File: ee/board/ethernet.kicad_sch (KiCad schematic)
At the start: 20 parts, among them J8 HR911105A, U1 RTL8201F, Y1 Crystal_GND24_Small

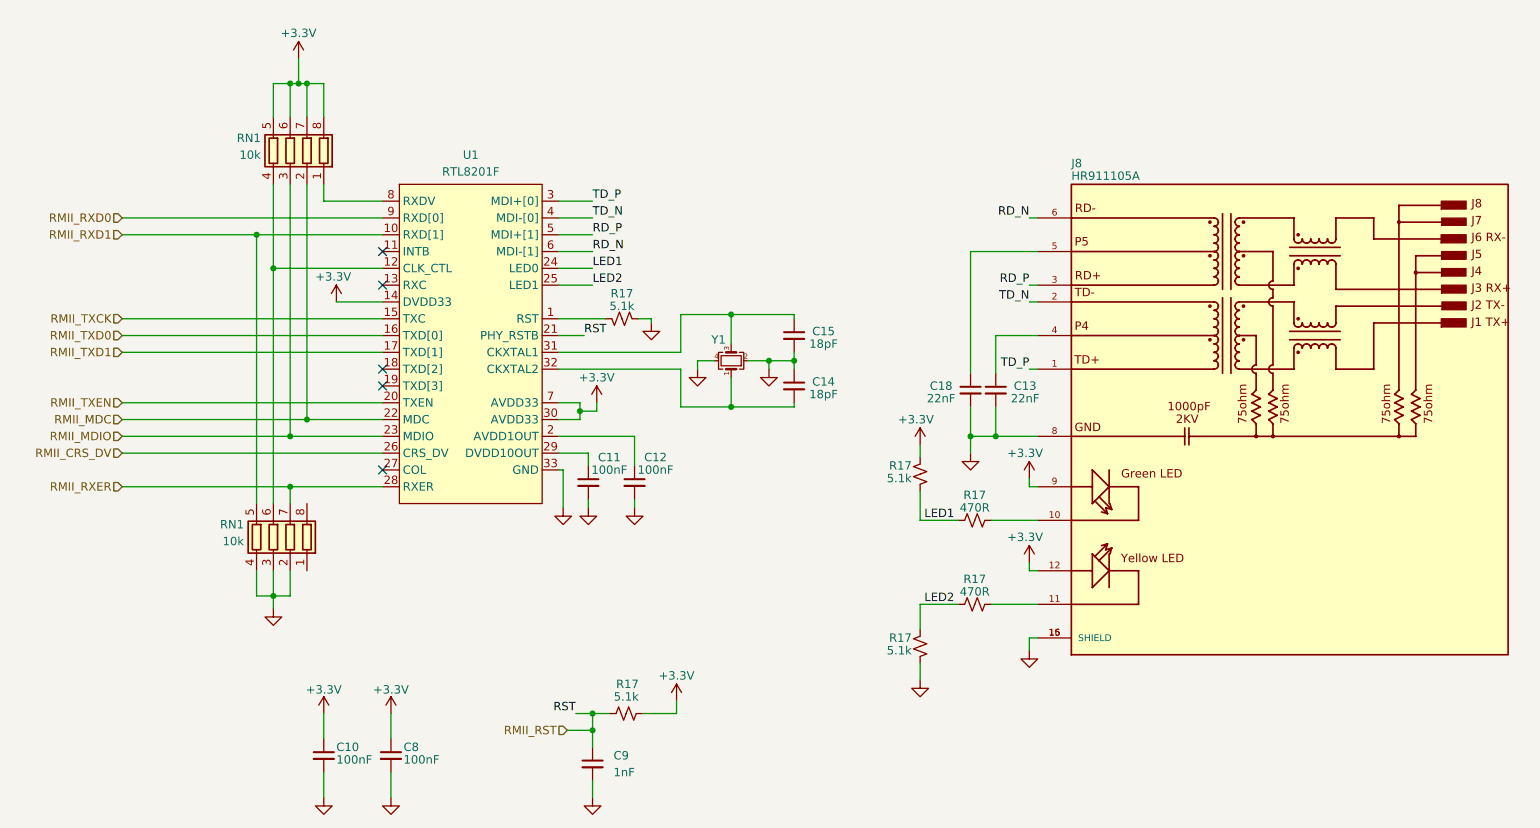
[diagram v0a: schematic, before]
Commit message: Nearly finished routing.
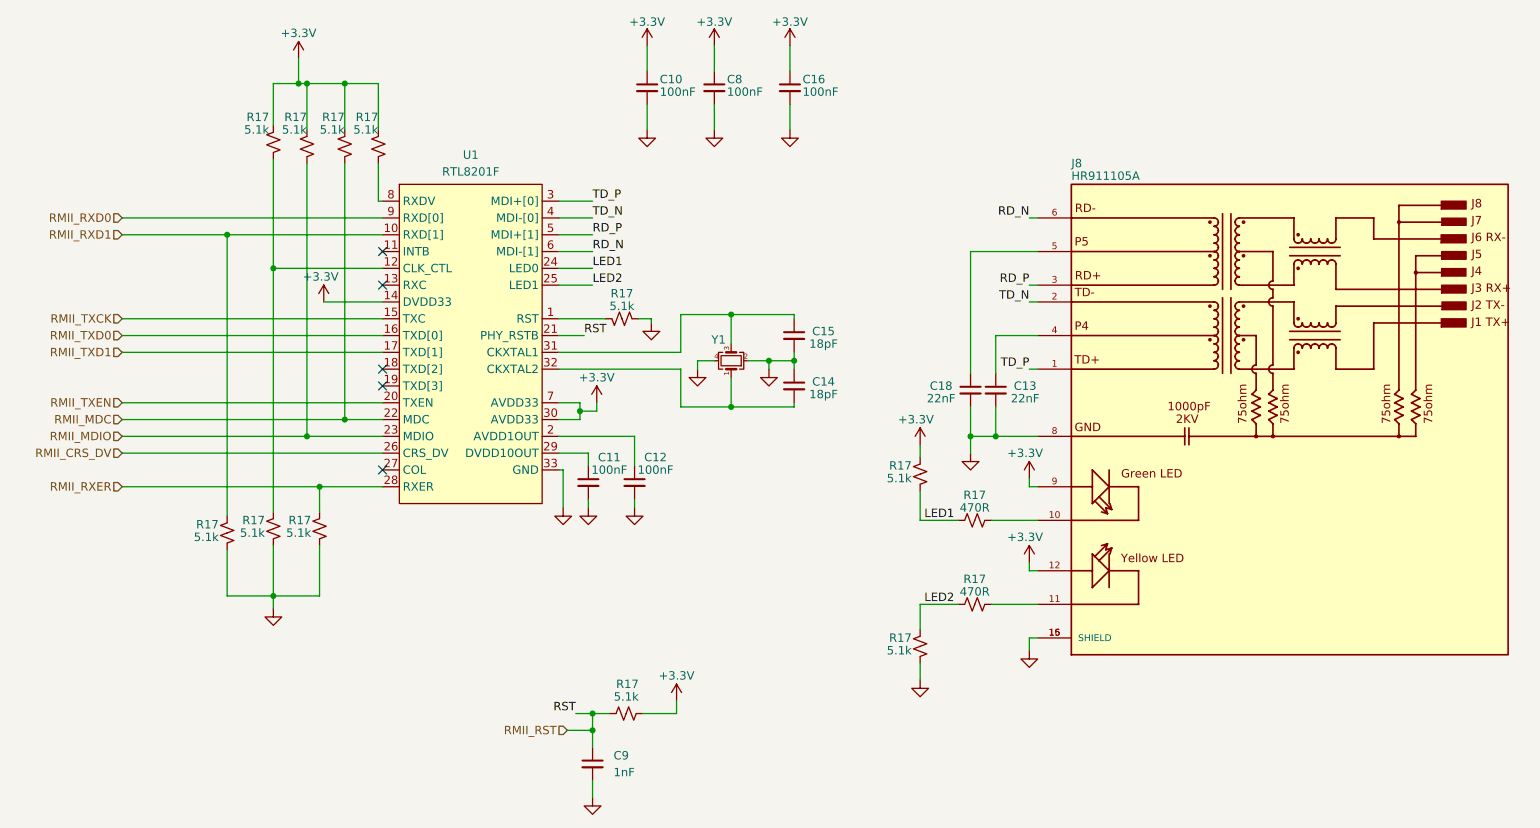
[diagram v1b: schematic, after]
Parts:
- removed RN1 (x2): 10k, Resistor_SMD:R_Array_Convex_4x0402, symbol Device:R_Pack04
- added C16: 100nF, Capacitor_SMD:C_0603_1608Metric, symbol Device:C_Small
- added R17 (x7): 5.1k, Resistor_SMD:R_0603_1608Metric, symbol Device:R_Small_US
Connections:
- net +3V3: now also C16.1, R17.2, R17.2, R17.2, R17.2
- net GND: now also C16.2, R17.1, R17.1, R17.1
- net RMII_MDC: now also R17.1
- net RMII_MDIO: now also R17.1
- net RMII_RXD1: now also R17.2
- net RMII_RXER: now also R17.2
- net at U1.12 (CLK_CTL): now also R17.1, R17.2
- net at U1.8 (RXDV): now also R17.1
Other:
- moved on the sheet: C10, C8

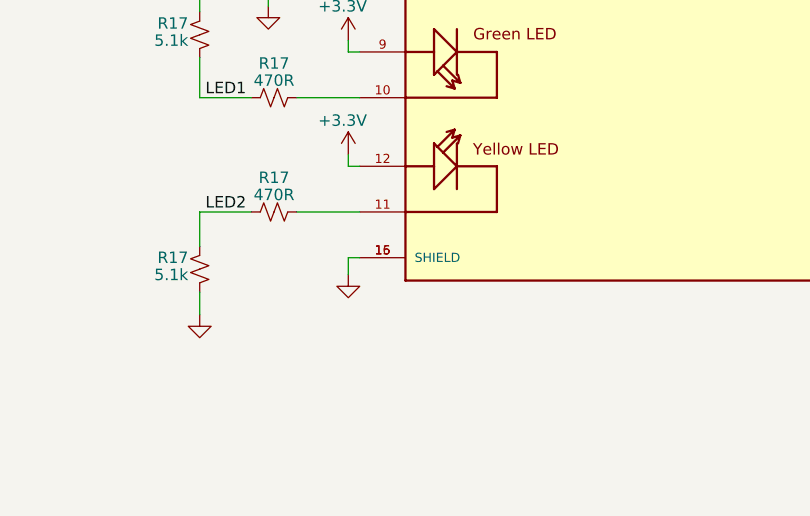
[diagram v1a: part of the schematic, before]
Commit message: Finished R1
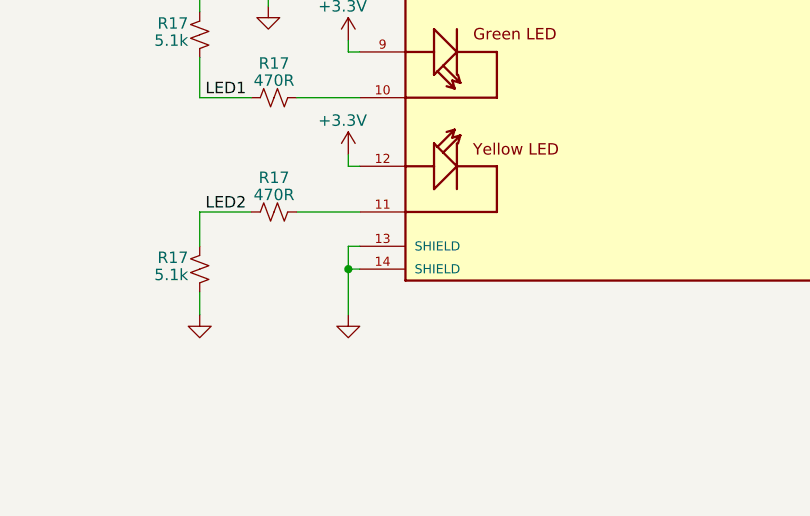
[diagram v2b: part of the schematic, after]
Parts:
- C10, C11, C12, C16, C8: MPN (none) -> CC0603KRX7R7BB104
- C14, C15: MPN (none) -> CC0603JPNPO9BN180
- R17: MPN (none) -> RC0603FR-135K1L
- R17: MPN (none) -> RC0603FR-13470KL
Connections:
- net GND: now also J8.13 (SHIELD), J8.14 (SHIELD); no longer J8.15 (SHIELD), J8.16 (SHIELD)
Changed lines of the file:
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@@
   (junction (at 86.995 90.17) (diameter 0) (color 0 0 0 0)
+  )
+  (junction (at 190.5 124.46) (diameter 0) (color 0 0 0 0)
   )
   (junction (at 83.185 100.33) (diameter 0) (color 0 0 0 0)
@@
     (stroke (width 0) (type default))
   )
+  (wire (pts (xy 190.5 121.92) (xy 190.5 124.46))
+    (stroke (width 0) (type default))
+  )
   (wire (pts (xy 181.61 92.71) (xy 185.42 92.71))
     (stroke (width 0) (type default))
@@
     (stroke (width 0) (type default))
   )
+  (wire (pts (xy 190.5 124.46) (xy 191.77 124.46))
+    (stroke (width 0) (type default))
+  )
   (wire (pts (xy 137.795 88.265) (xy 145.415 88.265))
     (stroke (width 0) (type default))
@@
     (stroke (width 0) (type default))
   )
-  (wire (pts (xy 190.5 125.095) (xy 190.5 123.19))
+  (wire (pts (xy 190.5 129.54) (xy 190.5 124.46))
     (stroke (width 0) (type default))
   )
@@
     (stroke (width 0) (type default))
   )
+  (wire (pts (xy 191.77 121.92) (xy 190.5 121.92))
+    (stroke (width 0) (type default))
+  )
   (wire (pts (xy 69.215 109.855) (xy 69.215 116.84))
     (stroke (width 0) (type default))
@@
   )
   (wire (pts (xy 137.795 74.295) (xy 145.415 74.295))
-    (stroke (width 0) (type default))
-  )
-  (wire (pts (xy 190.5 123.19) (xy 191.77 123.19))
     (stroke (width 0) (type default))
   )
@@
     (pin "11")
     (pin "12")
-    (pin "15")
-    (pin "16")
     (pin "2")
     (pin "3")
@@
     (pin "8")
     (pin "9")
+    (pin "13")
+    (pin "14")
     (instances
       (project "board"
@@
     )
     (property "Datasheet" "~" (at 173.99 124.46 0)
+      (effects (font (size 1.27 1.27)) hide)
+    )
+    (property "MPN" "RC0603FR-135K1L" (at 173.99 124.46 0)
       (effects (font (size 1.27 1.27)) hide)
     )
@@
     )
   )
-  (symbol (lib_id "power:GND") (at 190.5 125.095 0) (unit 1)
+  (symbol (lib_id "power:GND") (at 190.5 129.54 0) (unit 1)
     (in_bom yes) (on_board yes) (dnp no) (fields_autoplaced)
-    (property "Reference" "#PWR030" (at 190.5 131.445 0)
-      (effects (font (size 1.27 1.27)) hide)
-    )
-    (property "Value" "GND" (at 190.5 129.5384 0)
-      (effects (font (size 1.27 1.27)) hide)
-    )
-    (property "Footprint" "" (at 190.5 125.095 0)
-      (effects (font (size 1.27 1.27)) hide)
-    )
-    (property "Datasheet" "" (at 190.5 125.095 0)
+    (property "Reference" "#PWR030" (at 190.5 135.89 0)
+      (effects (font (size 1.27 1.27)) hide)
+    )
+    (property "Value" "GND" (at 190.5 133.9834 0)
+      (effects (font (size 1.27 1.27)) hide)
+    )
+    (property "Footprint" "" (at 190.5 129.54 0)
+      (effects (font (size 1.27 1.27)) hide)
+    )
+    (property "Datasheet" "" (at 190.5 129.54 0)
       (effects (font (size 1.27 1.27)) hide)
     )
@@
       (effects (font (size 1.27 1.27)) hide)
     )
+    (property "MPN" "CC0603KRX7R7BB104" (at 154.305 40.005 0)
+      (effects (font (size 1.27 1.27)) hide)
+    )
     (pin "1")
     (pin "2")
@@
       (effects (font (size 1.27 1.27)) hide)
     )
+    (property "MPN" "CC0603JPNPO9BN180" (at 154.94 85.09 0)
+      (effects (font (size 1.27 1.27)) hide)
+    )
     (pin "1")
     (pin "2")
@@
     )
     (property "Datasheet" "~" (at 182.245 118.11 0)
+      (effects (font (size 1.27 1.27)) hide)
+    )
+    (property "MPN" "RC0603FR-13470KL" (at 182.245 118.11 90)
       (effects (font (size 1.27 1.27)) hide)
     )
@@
     )
     (property "Datasheet" "~" (at 132.715 40.005 0)
+      (effects (font (size 1.27 1.27)) hide)
+    )
+    (property "MPN" "CC0603KRX7R7BB104" (at 132.715 40.005 0)
       (effects (font (size 1.27 1.27)) hide)
     )
@@
       (effects (font (size 1.27 1.27)) hide)
     )
+    (property "MPN" "RC0603FR-135K1L" (at 128.905 74.93 90)
+      (effects (font (size 1.27 1.27)) hide)
+    )
     (pin "1")
     (pin "2")
@@
     )
     (property "Datasheet" "~" (at 173.99 98.425 0)
+      (effects (font (size 1.27 1.27)) hide)
+    )
+    (property "MPN" "RC0603FR-135K1L" (at 173.99 98.425 0)
       (effects (font (size 1.27 1.27)) hide)
     )
@@
       (effects (font (size 1.27 1.27)) hide)
     )
+    (property "MPN" "RC0603FR-135K1L" (at 92.075 48.895 0)
+      (effects (font (size 1.27 1.27)) hide)
+    )
     (pin "1")
     (pin "2")
@@
       (effects (font (size 1.27 1.27)) hide)
     )
+    (property "MPN" "RC0603FR-135K1L" (at 76.2 48.26 0)
+      (effects (font (size 1.27 1.27)) hide)
+    )
     (pin "1")
     (pin "2")
@@
     )
     (property "Datasheet" "~" (at 130.81 99.695 0)
+      (effects (font (size 1.27 1.27)) hide)
+    )
+    (property "MPN" "CC0603KRX7R7BB104" (at 130.81 99.695 0)
       (effects (font (size 1.27 1.27)) hide)
     )
@@
       (effects (font (size 1.27 1.27)) hide)
     )
+    (property "MPN" "RC0603FR-135K1L" (at 76.2 106.68 0)
+      (effects (font (size 1.27 1.27)) hide)
+    )
     (pin "1")
     (pin "2")
@@
       (effects (font (size 1.27 1.27)) hide)
     )
+    (property "MPN" "CC0603JPNPO9BN180" (at 154.94 77.47 0)
+      (effects (font (size 1.27 1.27)) hide)
+    )
     (pin "1")
     (pin "2")
@@
       (effects (font (size 1.27 1.27)) hide)
     )
+    (property "MPN" "CC0603KRX7R7BB104" (at 142.875 40.005 0)
+      (effects (font (size 1.27 1.27)) hide)
+    )
     (pin "1")
     (pin "2")
@@
     )
     (property "Datasheet" "~" (at 83.185 106.68 0)
+      (effects (font (size 1.27 1.27)) hide)
+    )
+    (property "MPN" "RC0603FR-135K1L" (at 83.185 106.68 0)
       (effects (font (size 1.27 1.27)) hide)
     )
@@
       (effects (font (size 1.27 1.27)) hide)
     )
+    (property "MPN" "RC0603FR-135K1L" (at 69.215 107.315 0)
+      (effects (font (size 1.27 1.27)) hide)
+    )
     (pin "1")
     (pin "2")
@@
     )
     (property "Datasheet" "~" (at 123.825 99.695 0)
+      (effects (font (size 1.27 1.27)) hide)
+    )
+    (property "MPN" "CC0603KRX7R7BB104" (at 123.825 99.695 0)
       (effects (font (size 1.27 1.27)) hide)
     )
@@
       (effects (font (size 1.27 1.27)) hide)
     )
+    (property "MPN" "RC0603FR-135K1L" (at 129.54 134.62 90)
+      (effects (font (size 1.27 1.27)) hide)
+    )
     (pin "1")
     (pin "2")
@@
       (effects (font (size 1.27 1.27)) hide)
     )
+    (property "MPN" "RC0603FR-135K1L" (at 81.28 48.895 0)
+      (effects (font (size 1.27 1.27)) hide)
+    )
     (pin "1")
     (pin "2")
@@
     )
     (property "Datasheet" "~" (at 182.245 105.41 0)
+      (effects (font (size 1.27 1.27)) hide)
+    )
+    (property "MPN" "RC0603FR-13470KL" (at 182.245 105.41 90)
       (effects (font (size 1.27 1.27)) hide)
     )
@@
       (effects (font (size 1.27 1.27)) hide)
     )
+    (property "MPN" "RC0603FR-135K1L" (at 86.995 48.895 0)
+      (effects (font (size 1.27 1.27)) hide)
+    )
